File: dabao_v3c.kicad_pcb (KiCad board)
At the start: 6 copper layers, 17.8 x 21.1 mm, 60 parts, among them J1 USB_C_Receptacle_USB2.0_16P, Q1 LP0404N3T5G, Q2 LN237N3T5G, SW1 SKTAAAE010, SW2 SKTAAAE010, U1 baochip1x, U3 SMD IC PMIC;DCDC Buck-ADJ-1A,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, U5 EMS4000RSW, U7 SGM40567-4.2XG/TR, U8 SX1801CCR, U9 SMD IC PMIC;DCDC Buck-ADJ-1A,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, Y2 48.000MHz

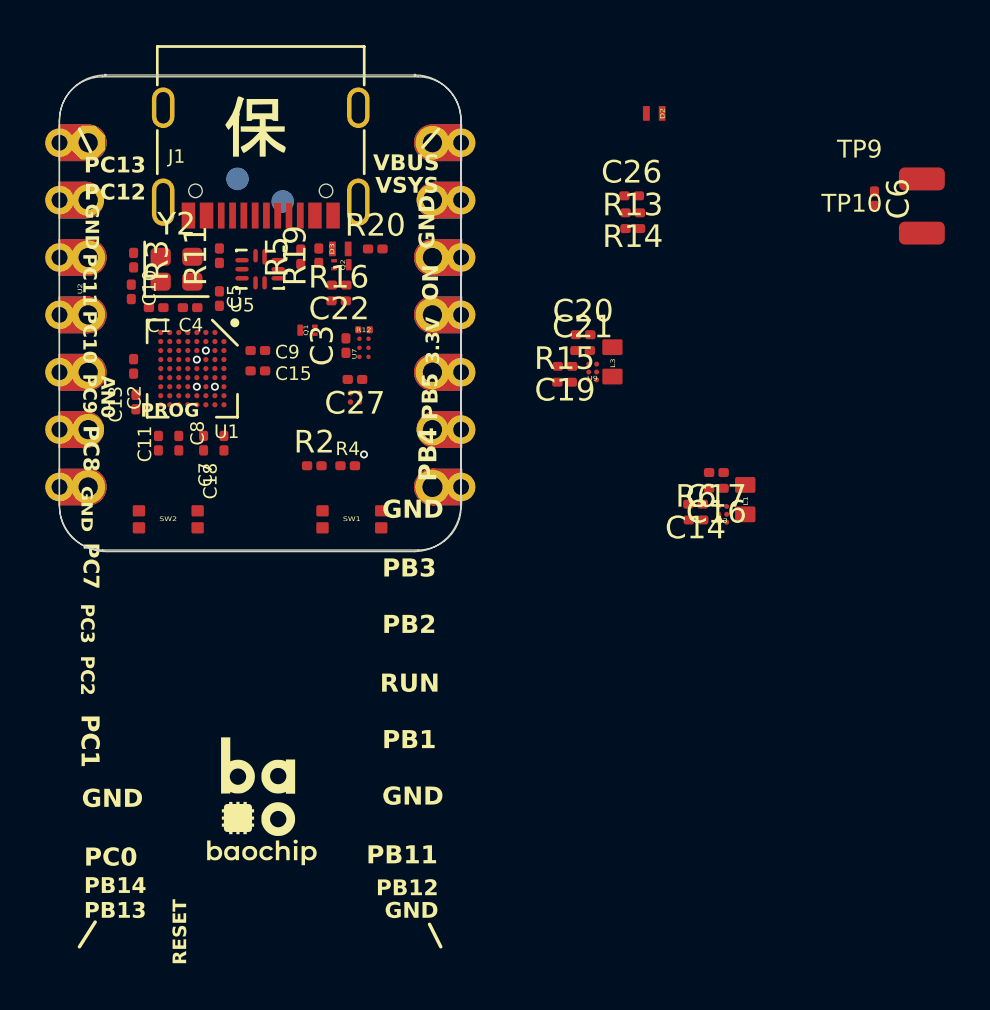
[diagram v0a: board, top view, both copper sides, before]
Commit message: tentative bao layout
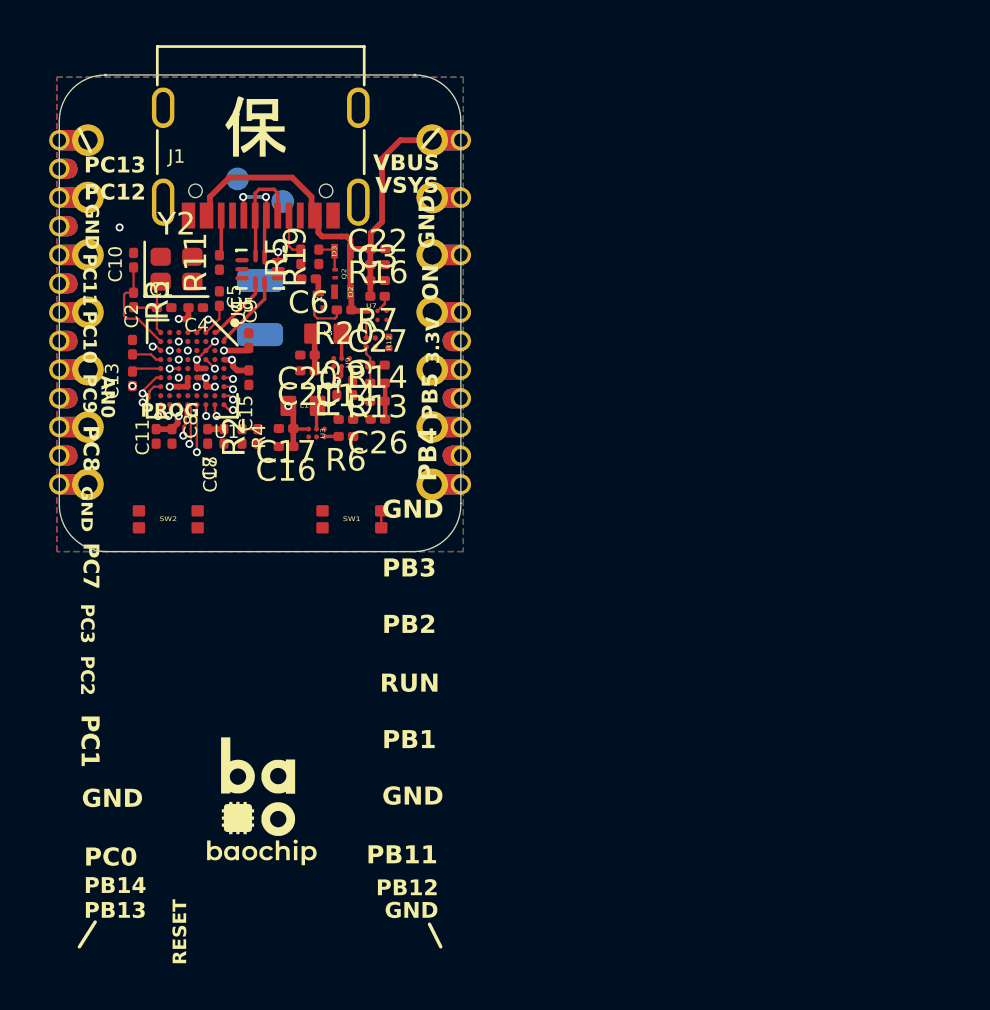
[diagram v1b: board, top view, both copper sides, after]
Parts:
- removed U2: ~, xiao:MOUDLE14P-XIAO-HALF-HOLE
- added R7: 5.1K, Resistor_SMD:R_0201_0603Metric, F.Cu at (137.2, 69.2)
- added U4: XIAO-HALF-HOLE-23P, xiao:MOUDLE23P-XIAO-HALF-HOLE, F.Cu at (132.0, 69.9)
- TP10, TP9: moved to B.Cu
- moved TP10 29.6 mm to (132.0, 70.9), turned to 180 degrees
- moved TP9 29.6 mm to (132.0, 68.5), turned to 180 degrees
- moved C6 25.3 mm to (134.2, 68.4), turned to 180 degrees
- moved L1 20.0 mm to (133.9, 74.0), turned to 180 degrees
- moved C17 19.1 mm to (133.2, 75.0)
- moved C16 19.1 mm to (133.2, 75.8)
- moved U3 18.3 mm to (134.5, 75.2), turned to 90 degrees
- moved R6 15.9 mm to (135.8, 75.4), turned to 180 degrees
- moved C14 15.9 mm to (135.8, 74.7), turned to 0 degrees
- moved D2 15.9 mm to (135.7, 69.0)
- moved C26 15.0 mm to (137.2, 74.6), turned to 180 degrees
- moved R14 14.0 mm to (137.2, 73.8), turned to 0 degrees
- moved R13 13.2 mm to (137.2, 73.0), turned to 180 degrees
- moved L3 12.7 mm to (134.9, 70.8), turned to 180 degrees
- moved C20 12.2 mm to (134.1, 71.8), turned to 180 degrees
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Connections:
- C16 pad 1: +3.3V -> +0.9V
- C17 pad 1: +3.3V -> +0.9V
- L1 pad 2: +3.3V -> +0.9V
- U1 pad B5: unconnected-(U1C-PB6-PadB5) -> /PA5
- U1 pad C4: GND -> /PA5
- U1 pad D7: +3.3V -> /PA7
- U1 pad E3: GND -> /PC5
- U1 pad E4: GND -> unconnected-(U1E-PF1-PadE4)
- U1 pad F2: unconnected-(U1E-PF8_PA1-PadF2) -> /PA1
- U1 pad F3: GND -> unconnected-(U1E-PA3-PadF3)
- U1 pad F4: GND -> /PC6
- U1 pad F6: +0.9V -> /PA6
- U1 pad G3: /PC9 -> /PA4
- U1 pad G5: unconnected-(U1E-PF4-PadG5) -> GND
- U1 pad G7: unconnected-(U1E-PF5-PadG7) -> +0.9V
- U3 pad A2: +3.3V -> +0.9V
- U7 pad B2: NCHG -> Net-(U7-NCHG)
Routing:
- net VBUS: track 0.00 -> 22.9 mm
- net /PC1: track 0.00 -> 16.5 mm, vias 0 -> 1
- net /PC2: track 0.00 -> 14.8 mm, vias 0 -> 1
- net /PB13: track 0.00 -> 14.4 mm, vias 0 -> 1
- net /PA4: track 0.00 -> 13.8 mm, vias 0 -> 1
- net /PC0: track 0.00 -> 12.7 mm, vias 0 -> 1
- net /PB2: track 0.00 -> 12.5 mm, vias 0 -> 1
- net /PC6: track 0.00 -> 12.1 mm, vias 0 -> 1
- net /PA1: track 0.00 -> 11.1 mm, vias 0 -> 2
- net /PA5: track 0.00 -> 11.0 mm, vias 0 -> 1
- net /PB1: track 0.00 -> 10.6 mm, vias 0 -> 1
- net /PC5: track 0.00 -> 10.1 mm, vias 0 -> 1
- net +0.9V: track 0.00 -> 9.93 mm, vias 0 -> 4
- net /PA6: track 0.00 -> 9.01 mm, vias 0 -> 1
- net /PA7: track 0.00 -> 7.87 mm, vias 0 -> 1
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- added copper zone on In3.Cu, net +3.3V
- added copper zone on B.Cu, net GND
- added copper zone on F.Cu, net GND
- added copper zone on In1.Cu, net GND

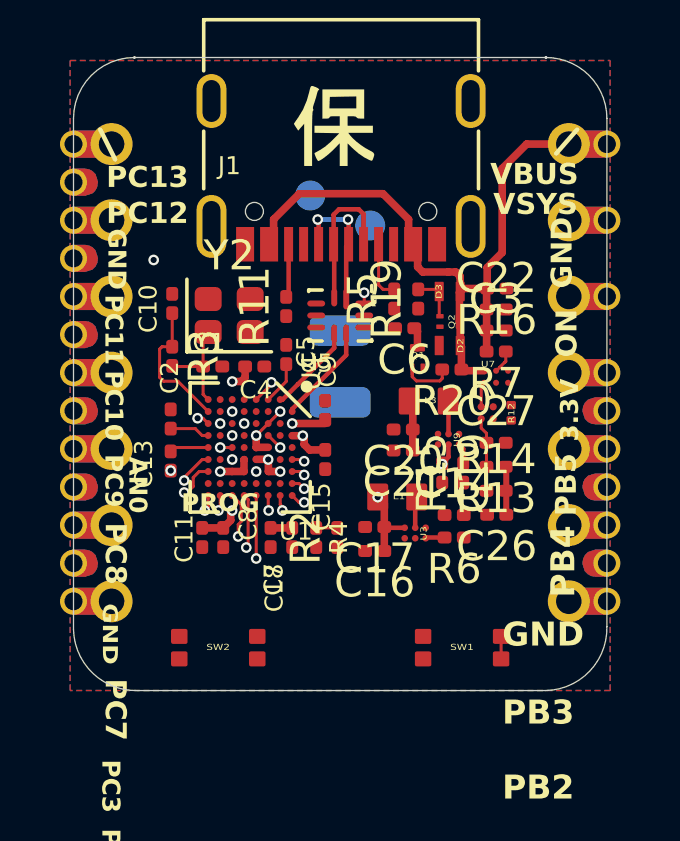
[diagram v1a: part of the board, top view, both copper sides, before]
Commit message: clean DRC v1
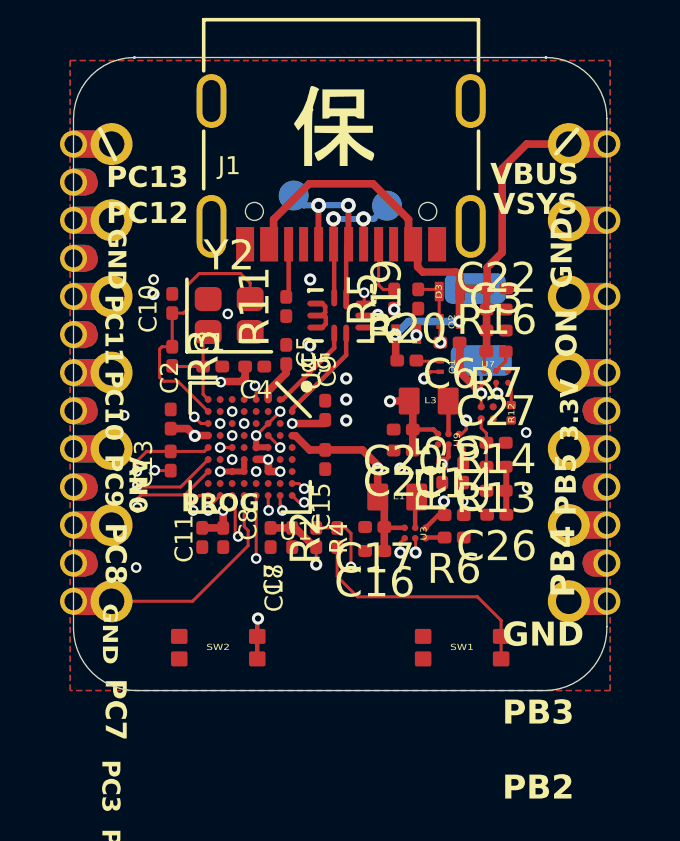
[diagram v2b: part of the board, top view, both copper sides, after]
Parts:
- moved TP10 5.89 mm to (136.5, 67.1), turned to 0 degrees
- moved TP9 4.81 mm to (136.7, 69.5)
- moved C6 1.58 mm to (135.7, 68.9)
- moved R20 1.53 mm to (134.2, 69.5), turned to 0 degrees
- moved D2 1.50 mm to (134.2, 68.6), turned to 180 degrees
- moved Q1 1.13 mm to (135.7, 69.7), turned to -90 degrees
- moved TP2 0.87 mm to (133.6, 64.3), turned to 90 degrees
- moved TP1 0.55 mm to (130.4, 64.0), turned to 90 degrees
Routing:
- net /RST_N: track 2.00 -> 15.4 mm, vias 0 -> 2
- net /PC13: track 5.51 -> 16.4 mm, vias 2 -> 3
- net Net-(SW1-B0): track 0.73 -> 8.31 mm
- net +3.3V: track 6.92 -> 12.0 mm, vias 4 -> 8
- net GND: track 2.33 -> 7.20 mm, vias 4 -> 19
- net /XO_48M: track 4.61 -> 8.88 mm
- net VSYS: track 0.73 -> 3.69 mm, vias 1 -> 6
- net VBUS: track 22.9 -> 25.7 mm, vias 0 -> 2
- net VBAT: track 1.53 -> 3.94 mm, vias 0 -> 1
- net /USBCONN_P: track 4.55 -> 6.68 mm
- net /PA4: track 13.8 -> 11.9 mm
- net /PC2: track 14.8 -> 16.5 mm
- net /PA1: track 11.1 -> 9.34 mm
- net /PA6: track 9.01 -> 10.7 mm
- net /PA7: track 7.87 -> 9.40 mm
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- added copper zone on In4.Cu, net +0.9V
- added copper zone on In2.Cu, net GND
- added copper zone on In3.Cu, net GND
- added copper zone on In4.Cu, net GND
- added copper zone on In4.Cu, net VSYS
